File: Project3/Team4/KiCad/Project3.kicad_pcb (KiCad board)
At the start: 2 copper layers, 88.9 x 43.2 mm, 18 parts, among them CON1 BARREL_JACK, P1 CONN_01X04, P2 CONN_01X17, Q1 MMBT3906, Q2 MMBT3906, SW1 Switch_SPDT_x2, SW2 Switch_SPDT_x2, SW3 SW_PUSH, U1 Teensy_3.1, U2 LM7805CT

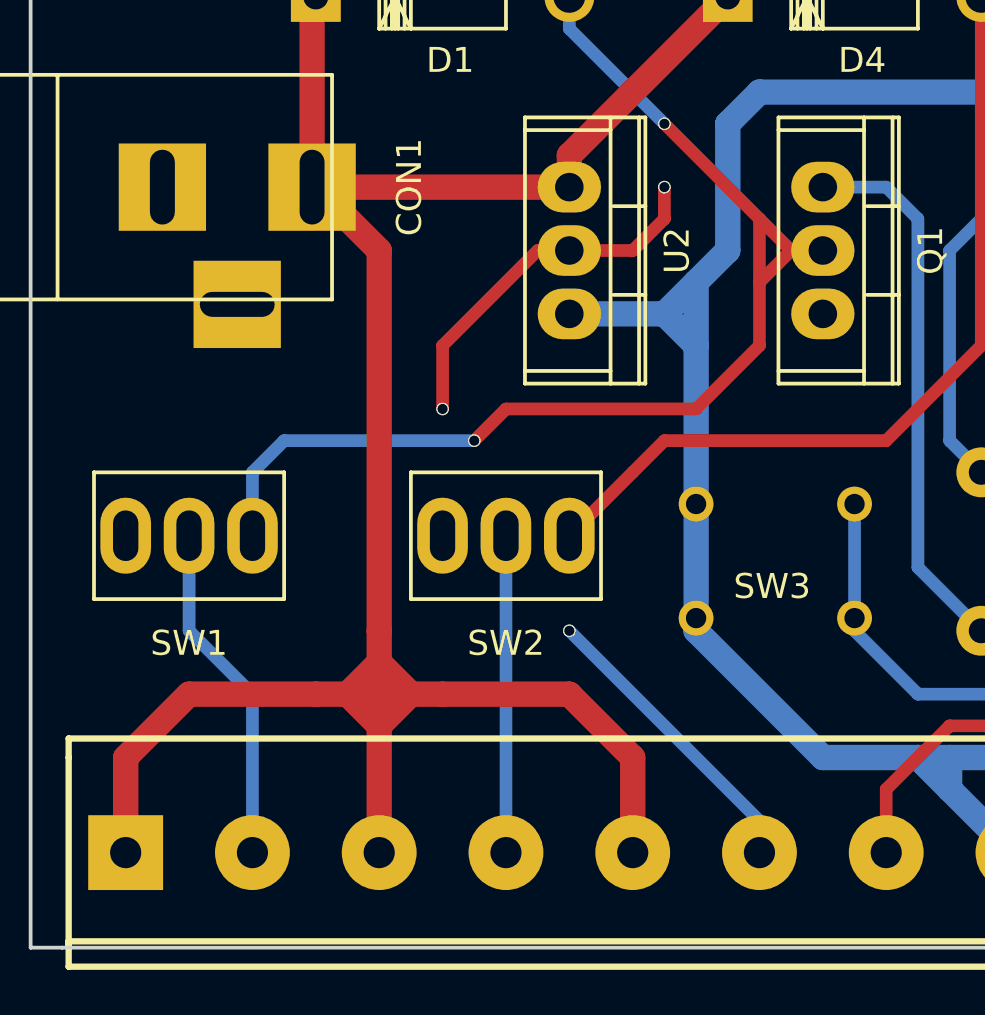
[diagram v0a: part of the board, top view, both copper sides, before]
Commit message: Updating proj 3 files
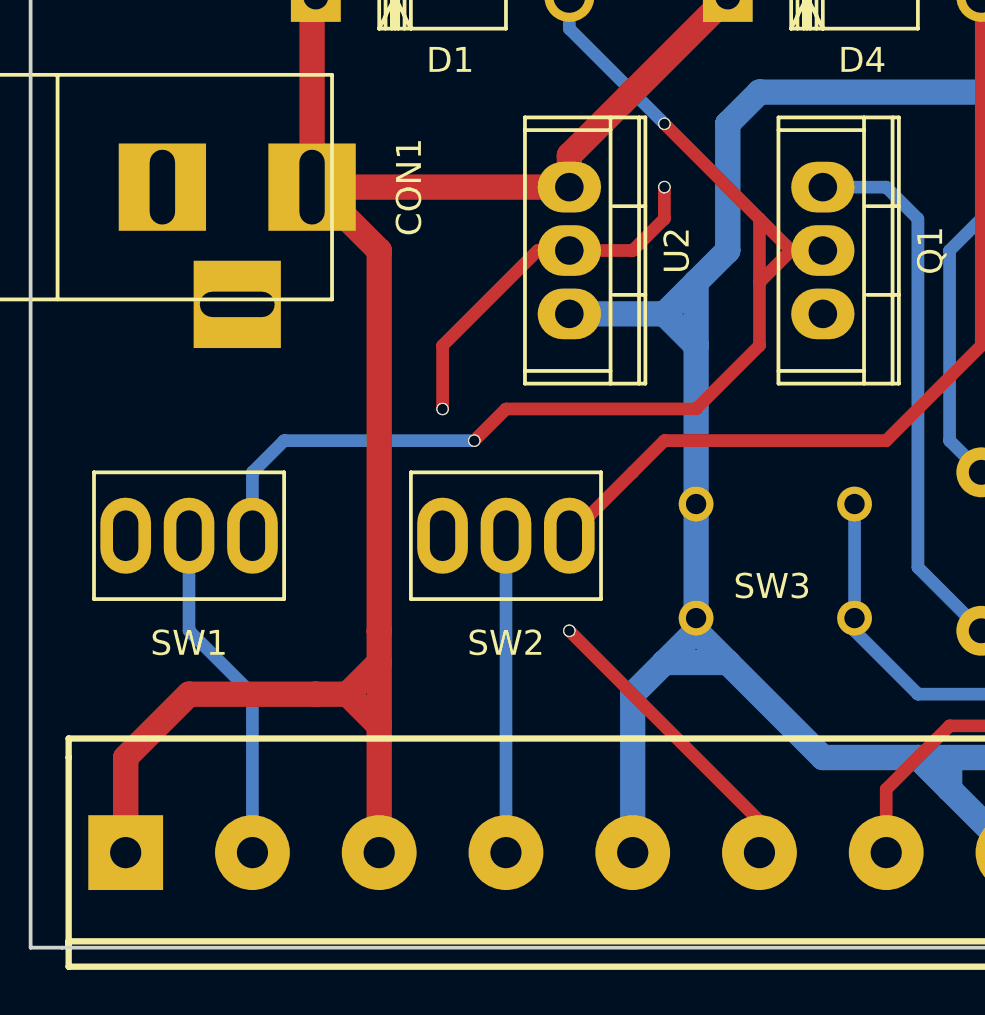
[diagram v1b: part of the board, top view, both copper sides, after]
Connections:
- P2 pad 5: +12V -> +5V
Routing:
- net +12V: track 93.3 -> 73.5 mm
- net +5V: track 122.3 -> 134.8 mm
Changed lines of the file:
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@@
     (links 48)
     (no_connects 0)
-    (area 106.604999 86.284999 195.655001 129.615001)
+    (area 86.944287 73.35 197.213 133.2992)
     (thickness 1.6)
     (drawings 8)
-    (tracks 161)
+    (tracks 159)
     (zones 0)
     (modules 18)
@@
     (mod_text_size 1 1)
     (mod_text_width 0.15)
-    (pad_size 2.032 2.54)
-    (pad_drill 1.143)
+    (pad_size 3.50012 3.50012)
+    (pad_drill 2.99974)
     (pad_to_mask_clearance 0.2)
     (aux_axis_origin 0 0)
     (visible_elements FFFFFF7F)
     (pcbplotparams
-      (layerselection 0x00030_80000001)
+      (layerselection 0x01000_80000001)
       (usegerberextensions false)
       (excludeedgelayer true)
@@
       (outputformat 1)
       (mirror false)
-      (drillshape 1)
+      (drillshape 0)
       (scaleselection 1)
       (outputdirectory ""))
@@
       (net 11 /Pump2GND))
     (pad 5 thru_hole circle (at -20.32 0) (size 2.99974 2.99974) (drill 1.24968) (layers *.Cu *.Mask F.SilkS)
-      (net 1 +12V))
+      (net 7 +5V))
     (pad 6 thru_hole circle (at -15.24 0) (size 2.99974 2.99974) (drill 1.24968) (layers *.Cu *.Mask F.SilkS)
       (net 2 Earth))
@@
     (fp_line (start 7.00024 4.50088) (end 7.00024 -4.50088) (layer F.SilkS) (width 0.15))
     (fp_line (start 7.00024 -4.50088) (end -7.50062 -4.50088) (layer F.SilkS) (width 0.15))
-    (pad 1 thru_hole rect (at 6.20014 0) (size 3.50012 3.50012) (drill oval 1.00076 2.99974) (layers *.Cu *.Mask F.SilkS)
+    (pad 1 thru_hole rect (at 6.20014 0) (size 3.50012 3.50012) (drill oval 1.016 2.99974) (layers *.Cu *.Mask F.SilkS)
       (net 1 +12V))
-    (pad 2 thru_hole rect (at 0.20066 0) (size 3.50012 3.50012) (drill oval 1.00076 2.99974) (layers *.Cu *.Mask F.SilkS)
-      (net 2 Earth))
-    (pad 3 thru_hole rect (at 3.2004 4.699) (size 3.50012 3.50012) (drill oval 2.99974 1.00076) (layers *.Cu *.Mask F.SilkS)
+    (pad 2 thru_hole rect (at 0.20066 0) (size 3.50012 3.50012) (drill oval 1.016 2.99974) (layers *.Cu *.Mask F.SilkS)
+      (net 2 Earth))
+    (pad 3 thru_hole rect (at 3.2004 4.699) (size 3.50012 3.50012) (drill oval 2.99974 1.016) (layers *.Cu *.Mask F.SilkS)
       (net 2 Earth))
   )
@@
   (gr_line (start 195.58 86.36) (end 195.58 129.54) (angle 90) (layer Edge.Cuts) (width 0.15))
   (gr_line (start 107.95 86.36) (end 195.58 86.36) (angle 90) (layer Edge.Cuts) (width 0.15))
-  (segment (start 120.65 120.65) (end 121.92 119.38) (width 1.016) (layer F.Cu) (net 1))
   (segment (start 119.38 119.38) (end 120.65 120.65) (width 1.016) (layer F.Cu) (net 1))
-  (segment (start 120.65 118.11) (end 121.92 119.38) (width 1.016) (layer F.Cu) (net 1))
   (segment (start 119.38 119.38) (end 120.65 118.11) (width 1.016) (layer F.Cu) (net 1))
   (segment (start 118.11 119.38) (end 119.38 119.38) (width 1.016) (layer F.Cu) (net 1))
-  (segment (start 119.38 119.38) (end 121.92 119.38) (width 1.016) (layer F.Cu) (net 1))
-  (segment (start 121.92 119.38) (end 123.19 119.38) (width 1.016) (layer F.Cu) (net 1))
-  (segment (start 130.81 121.92) (end 130.81 125.73) (width 1.016) (layer F.Cu) (net 1))
-  (segment (start 123.19 119.38) (end 128.27 119.38) (width 1.016) (layer F.Cu) (net 1))
-  (segment (start 128.27 119.38) (end 130.81 121.92) (width 1.016) (layer F.Cu) (net 1))
   (segment (start 110.49 125.73) (end 110.49 121.92) (width 1.016) (layer F.Cu) (net 1))
   (segment (start 113.03 119.38) (end 118.11 119.38) (width 1.016) (layer F.Cu) (net 1))
@@
   (segment (start 117.96014 99.06) (end 117.96014 91.58732) (width 1.016) (layer F.Cu) (net 1))
   (segment (start 117.96014 91.58732) (end 118.11 91.43746) (width 1.016) (layer F.Cu) (net 1))
-  (segment (start 135.89 125.73) (end 135.89 124.46) (width 0.508) (layer B.Cu) (net 2))
-  (segment (start 135.89 124.46) (end 128.27 116.84) (width 0.508) (layer B.Cu) (net 2))
+  (segment (start 135.89 125.73) (end 135.89 124.46) (width 0.508) (layer F.Cu) (net 2))
+  (segment (start 135.89 124.46) (end 128.27 116.84) (width 0.508) (layer F.Cu) (net 2))
   (via (at 128.27 116.84) (size 0.508) (drill 0.4064) (layers F.Cu B.Cu) (net 2))
   (segment (start 128.27 101.6) (end 127 101.6) (width 0.508) (layer F.Cu) (net 2))
@@
   (segment (start 144.78 102.87) (end 146.05 101.6) (width 0.508) (layer F.Cu) (net 6))
   (segment (start 144.78 91.43746) (end 144.78 100.33) (width 0.508) (layer F.Cu) (net 6))
+  (segment (start 132.08 118.11) (end 134.62 118.11) (width 1.016) (layer B.Cu) (net 7))
   (segment (start 133.35 116.332) (end 133.35 116.84) (width 1.016) (layer B.Cu) (net 7))
-  (segment (start 133.35 116.84) (end 138.43 121.92) (width 1.016) (layer B.Cu) (net 7))
+  (segment (start 133.35 116.84) (end 132.08 118.11) (width 1.016) (layer B.Cu) (net 7))
+  (segment (start 132.08 118.11) (end 130.81 119.38) (width 1.016) (layer B.Cu) (net 7))
+  (segment (start 130.81 119.38) (end 130.81 125.73) (width 1.016) (layer B.Cu) (net 7))
+  (segment (start 133.35 116.84) (end 134.62 118.11) (width 1.016) (layer B.Cu) (net 7))
+  (segment (start 134.62 118.11) (end 138.43 121.92) (width 1.016) (layer B.Cu) (net 7))
   (segment (start 138.43 121.92) (end 142.24 121.92) (width 1.016) (layer B.Cu) (net 7))
   (segment (start 133.35 111.76) (end 133.35 116.332) (width 1.016) (layer B.Cu) (net 7))
